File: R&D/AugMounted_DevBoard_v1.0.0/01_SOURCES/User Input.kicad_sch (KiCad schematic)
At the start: 24 parts, among them J501 J_0788641001_PAD, J502 J_0788641001, J503 J_0788641001, J504 J_0788641001_PAD, SW501 SW_SKRTLAE010, U502 MP34DT05TR-A

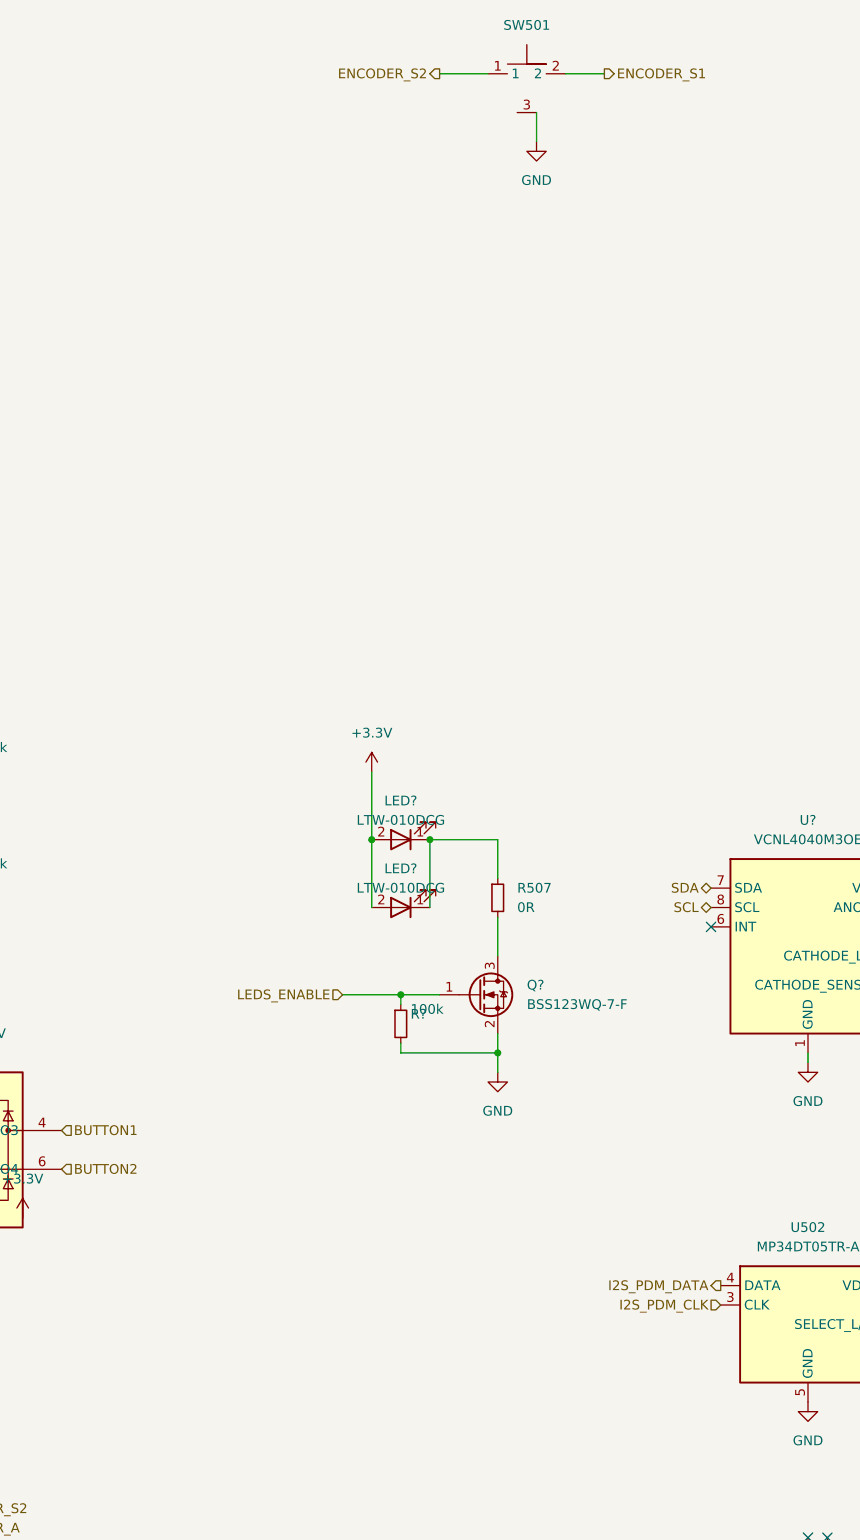
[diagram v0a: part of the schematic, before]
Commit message: Layout almost done
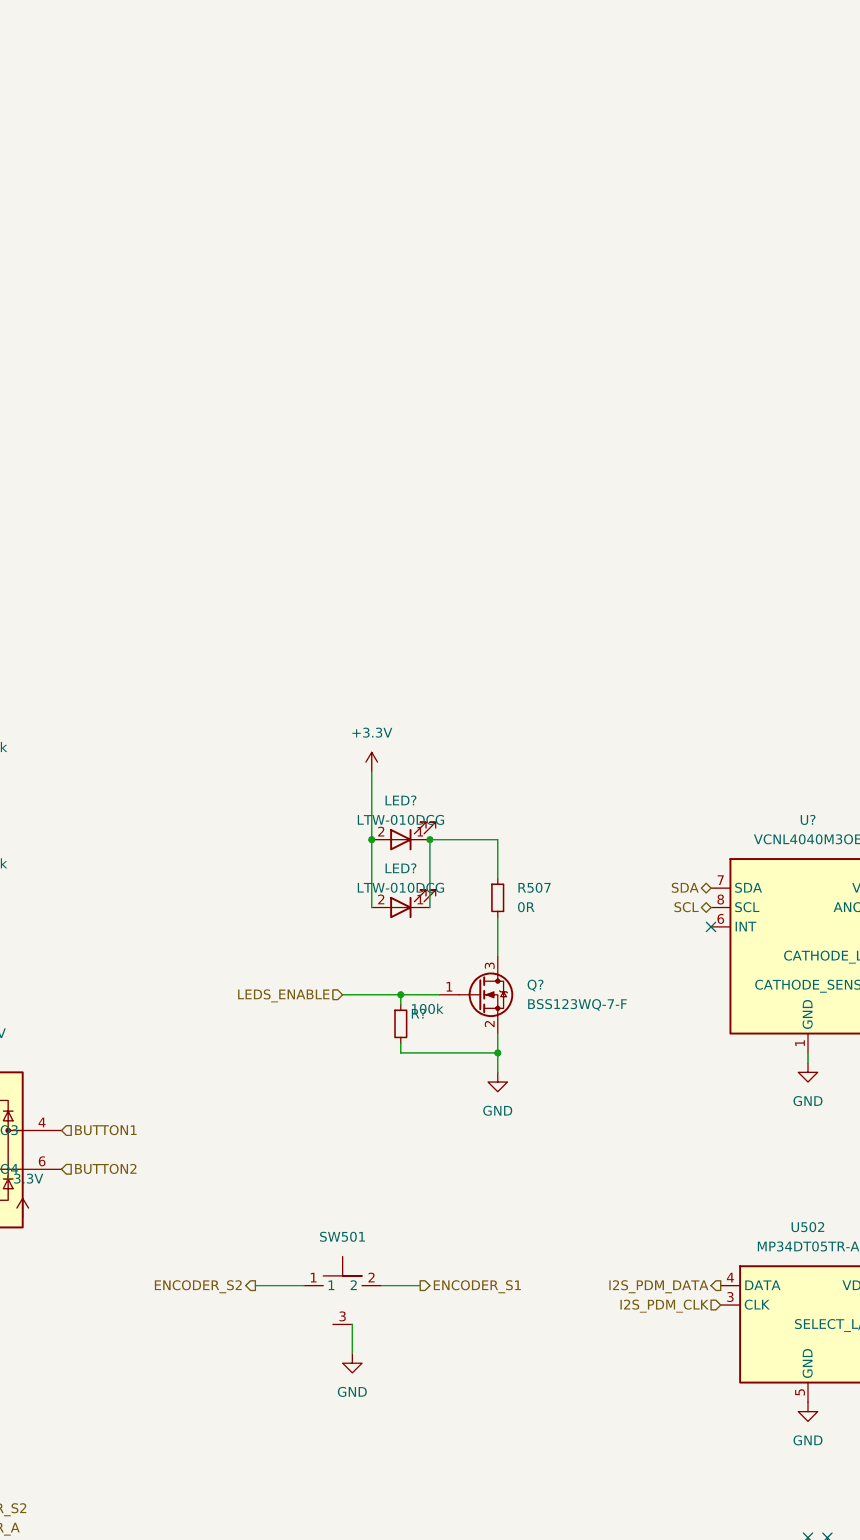
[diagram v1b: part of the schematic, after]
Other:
- moved on the sheet: SW501
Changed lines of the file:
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@@
     (stroke (width 0) (type default))
   )
-  (wire (pts (xy 175.26 -49.53) (xy 175.26 -53.34))
+  (wire (pts (xy 151.13 109.22) (xy 151.13 105.41))
     (stroke (width 0) (type default))
   )
@@
     (stroke (width 0) (type default))
   )
-  (wire (pts (xy 162.56 -58.42) (xy 168.91 -58.42))
+  (wire (pts (xy 138.43 100.33) (xy 144.78 100.33))
     (stroke (width 0) (type default))
   )
-  (wire (pts (xy 184.15 -58.42) (xy 179.07 -58.42))
+  (wire (pts (xy 160.02 100.33) (xy 154.94 100.33))
     (stroke (width 0) (type default))
   )
@@
     (effects (font (size 1.27 1.27)) (justify left))
   )
-  (hierarchical_label "ENCODER_S2" (shape output) (at 162.56 -58.42 180) (fields_autoplaced)
+  (hierarchical_label "ENCODER_S2" (shape output) (at 138.43 100.33 180) (fields_autoplaced)
     (effects (font (size 1.27 1.27)) (justify right))
   )
@@
     (effects (font (size 1.27 1.27)) (justify right))
   )
-  (hierarchical_label "ENCODER_S1" (shape output) (at 184.15 -58.42 0) (fields_autoplaced)
+  (hierarchical_label "ENCODER_S1" (shape output) (at 160.02 100.33 0) (fields_autoplaced)
     (effects (font (size 1.27 1.27)) (justify left))
   )
@@
     )
   )
-  (symbol (lib_id "power:GND") (at 175.26 -49.53 0) (unit 1)
+  (symbol (lib_id "power:GND") (at 151.13 109.22 0) (unit 1)
     (in_bom yes) (on_board yes) (dnp no)
-    (property "Reference" "#PWR0518" (at 175.26 -43.18 0)
-      (effects (font (size 1.27 1.27)) hide)
-    )
-    (property "Value" "GND" (at 175.26 -44.45 0)
-      (effects (font (size 1.27 1.27)))
-    )
-    (property "Footprint" "" (at 175.26 -49.53 0)
-      (effects (font (size 1.27 1.27)) hide)
-    )
-    (property "Datasheet" "" (at 175.26 -49.53 0)
+    (property "Reference" "#PWR0518" (at 151.13 115.57 0)
+      (effects (font (size 1.27 1.27)) hide)
+    )
+    (property "Value" "GND" (at 151.13 114.3 0)
+      (effects (font (size 1.27 1.27)))
+    )
+    (property "Footprint" "" (at 151.13 109.22 0)
+      (effects (font (size 1.27 1.27)) hide)
+    )
+    (property "Datasheet" "" (at 151.13 109.22 0)
       (effects (font (size 1.27 1.27)) hide)
     )
@@
     )
   )
-  (symbol (lib_id ".mounted-lib:SW_SKRTLAE010") (at 173.99 -59.69 0) (unit 1)
-    (in_bom yes) (on_board yes) (dnp no) (fields_autoplaced)
-    (property "Reference" "SW501" (at 173.99 -64.77 0)
-      (effects (font (size 1.27 1.27)))
-    )
-    (property "Value" "SW_SKRTLAE010" (at 190.5 -72.39 0)
-      (effects (font (size 1.27 1.27)) (justify left) hide)
-    )
-    (property "Footprint" ".mounted-lib:SW_SKRTLAE010" (at 190.5 -49.276 0)
-      (effects (font (size 1.27 1.27)) (justify left) hide)
-    )
-    (property "Datasheet" "https://datasheet.lcsc.com/lcsc/1809191932_ALPSALPINE-SKRTLAE010_C110293.pdf" (at 190.5 -47.371 0)
-      (effects (font (size 1.27 1.27)) (justify left) hide)
-    )
-    (property "Manufacturer" "ALPS ALPINE" (at 190.5 -45.466 0)
-      (effects (font (size 1.27 1.27)) (justify left) hide)
-    )
-    (property "MPN" "SKRTLAE010" (at 190.5 -42.926 0)
-      (effects (font (size 1.27 1.27)) (justify left) hide)
-    )
-    (property "DisplayValue" "SKRTLAE010" (at 167.64 -55.88 0)
-      (effects (font (size 1.27 1.27)) (justify left) hide)
-    )
-    (property "CMP_ID" "1084" (at 190.5 -70.485 0)
-      (effects (font (size 1.27 1.27)) (justify left) hide)
-    )
-    (property "Category" "ELECTROMECHANICAL" (at 190.5 -68.58 0)
-      (effects (font (size 1.27 1.27)) (justify left) hide)
-    )
-    (property "Family" "TACTILE SWITCH" (at 190.5 -66.675 0)
-      (effects (font (size 1.27 1.27)) (justify left) hide)
-    )
-    (property "_Created" "JCN 2023-11-16" (at 190.5 -64.77 0)
-      (effects (font (size 1.27 1.27)) (justify left) hide)
-    )
-    (property "_Checked" "" (at 190.5 -62.992 0)
-      (effects (font (size 1.27 1.27)) (justify left) hide)
-    )
-    (property "_Confirmed" "" (at 190.5 -60.96 0)
-      (effects (font (size 1.27 1.27)) (justify left) hide)
-    )
-    (property "Mount" "SMD" (at 190.5 -61.341 0)
-      (effects (font (size 1.27 1.27)) (justify left) hide)
-    )
-    (property "Package" "RIGHT ANGLE" (at 190.5 -40.64 0)
-      (effects (font (size 1.27 1.27)) (justify left) hide)
-    )
-    (property "PartStatus" "L3360" (at 190.5 -59.055 0)
-      (effects (font (size 1.27 1.27)) (justify left) hide)
-    )
-    (property "TempMin_C" "-30°C" (at 190.5 -56.896 0)
-      (effects (font (size 1.27 1.27)) (justify left) hide)
-    )
-    (property "TempMax_C" "85°C" (at 190.5 -54.991 0)
-      (effects (font (size 1.27 1.27)) (justify left) hide)
-    )
-    (property "Automotive" "N" (at 190.5 -53.086 0)
-      (effects (font (size 1.27 1.27)) (justify left) hide)
-    )
-    (property "MaxHeight_mm" "3.3mm" (at 190.5 -51.181 0)
-      (effects (font (size 1.27 1.27)) (justify left) hide)
-    )
+  (symbol (lib_id ".mounted-lib:SW_SKRTLAE010") (at 149.86 99.06 0) (unit 1)
+    (in_bom yes) (on_board yes) (dnp no) (fields_autoplaced)
+    (property "Reference" "SW501" (at 149.86 93.98 0)
+      (effects (font (size 1.27 1.27)))
+    )
+    (property "Value" "SW_SKRTLAE010" (at 166.37 86.36 0)
+      (effects (font (size 1.27 1.27)) (justify left) hide)
+    )
+    (property "Footprint" ".mounted-lib:SW_SKRTLAE010" (at 166.37 109.474 0)
+      (effects (font (size 1.27 1.27)) (justify left) hide)
+    )
+    (property "Datasheet" "https://datasheet.lcsc.com/lcsc/1809191932_ALPSALPINE-SKRTLAE010_C110293.pdf" (at 166.37 111.379 0)
+      (effects (font (size 1.27 1.27)) (justify left) hide)
+    )
+    (property "Manufacturer" "ALPS ALPINE" (at 166.37 113.284 0)
+      (effects (font (size 1.27 1.27)) (justify left) hide)
+    )
+    (property "MPN" "SKRTLAE010" (at 166.37 115.824 0)
+      (effects (font (size 1.27 1.27)) (justify left) hide)
+    )
+    (property "DisplayValue" "SKRTLAE010" (at 143.51 102.87 0)
+      (effects (font (size 1.27 1.27)) (justify left) hide)
+    )
+    (property "CMP_ID" "1084" (at 166.37 88.265 0)
+      (effects (font (size 1.27 1.27)) (justify left) hide)
+    )
+    (property "Category" "ELECTROMECHANICAL" (at 166.37 90.17 0)
+      (effects (font (size 1.27 1.27)) (justify left) hide)
+    )
+    (property "Family" "TACTILE SWITCH" (at 166.37 92.075 0)
+      (effects (font (size 1.27 1.27)) (justify left) hide)
+    )
+    (property "_Created" "JCN 2023-11-16" (at 166.37 93.98 0)
+      (effects (font (size 1.27 1.27)) (justify left) hide)
+    )
+    (property "_Checked" "" (at 166.37 95.758 0)
+      (effects (font (size 1.27 1.27)) (justify left) hide)
+    )
+    (property "_Confirmed" "" (at 166.37 97.79 0)
+      (effects (font (size 1.27 1.27)) (justify left) hide)
+    )
+    (property "Mount" "SMD" (at 166.37 97.409 0)
+      (effects (font (size 1.27 1.27)) (justify left) hide)
+    )
+    (property "Package" "RIGHT ANGLE" (at 166.37 118.11 0)
+      (effects (font (size 1.27 1.27)) (justify left) hide)
+    )
+    (property "PartStatus" "L3360" (at 166.37 99.695 0)
+      (effects (font (size 1.27 1.27)) (justify left) hide)
+    )
+    (property "TempMin_C" "-30°C" (at 166.37 101.854 0)
+      (effects (font (size 1.27 1.27)) (justify left) hide)
+    )
+    (property "TempMax_C" "85°C" (at 166.37 103.759 0)
+      (effects (font (size 1.27 1.27)) (justify left) hide)
+    )
+    (property "Automotive" "N" (at 166.37 105.664 0)
+      (effects (font (size 1.27 1.27)) (justify left) hide)
+    )
+    (property "MaxHeight_mm" "3.3mm" (at 166.37 107.569 0)
+      (effects (font (size 1.27 1.27)) (justify left) hide)
+    )
